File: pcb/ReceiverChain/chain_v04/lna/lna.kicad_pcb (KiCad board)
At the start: 2 copper layers, 40.4 x 15 mm, 17 parts, among them J1 RF-IN, J2 RF-OUT, U1 SKY67159, U2 TPS79933

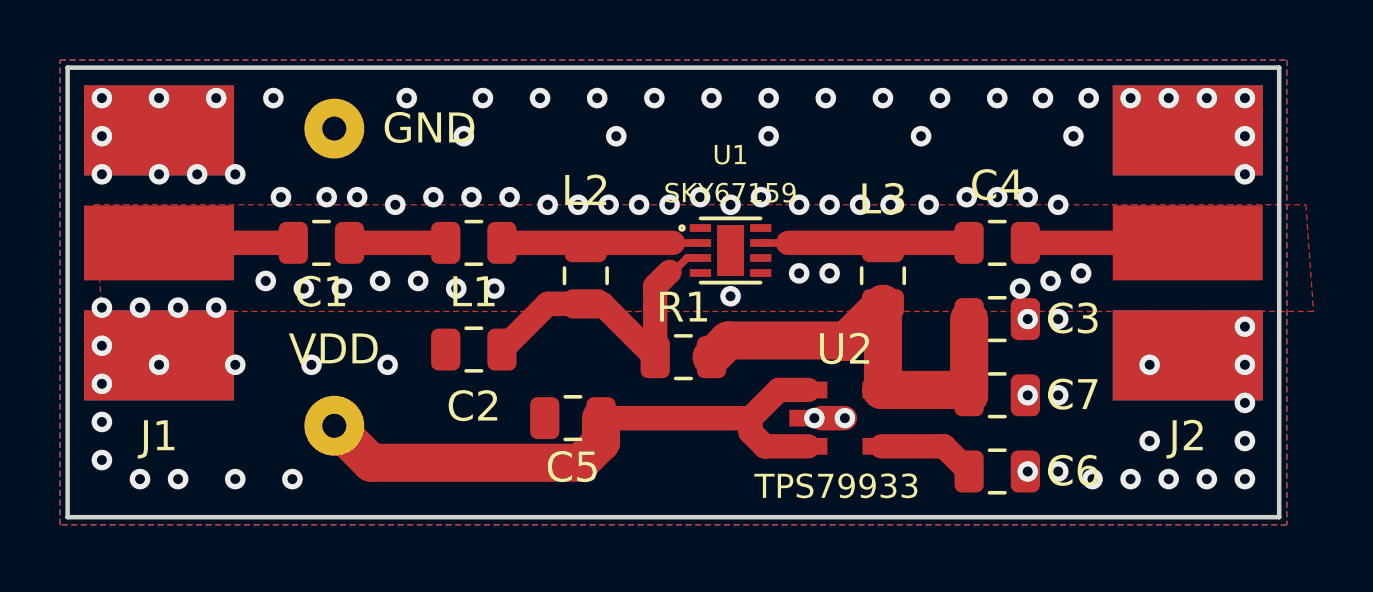
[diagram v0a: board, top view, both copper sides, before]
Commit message: saving
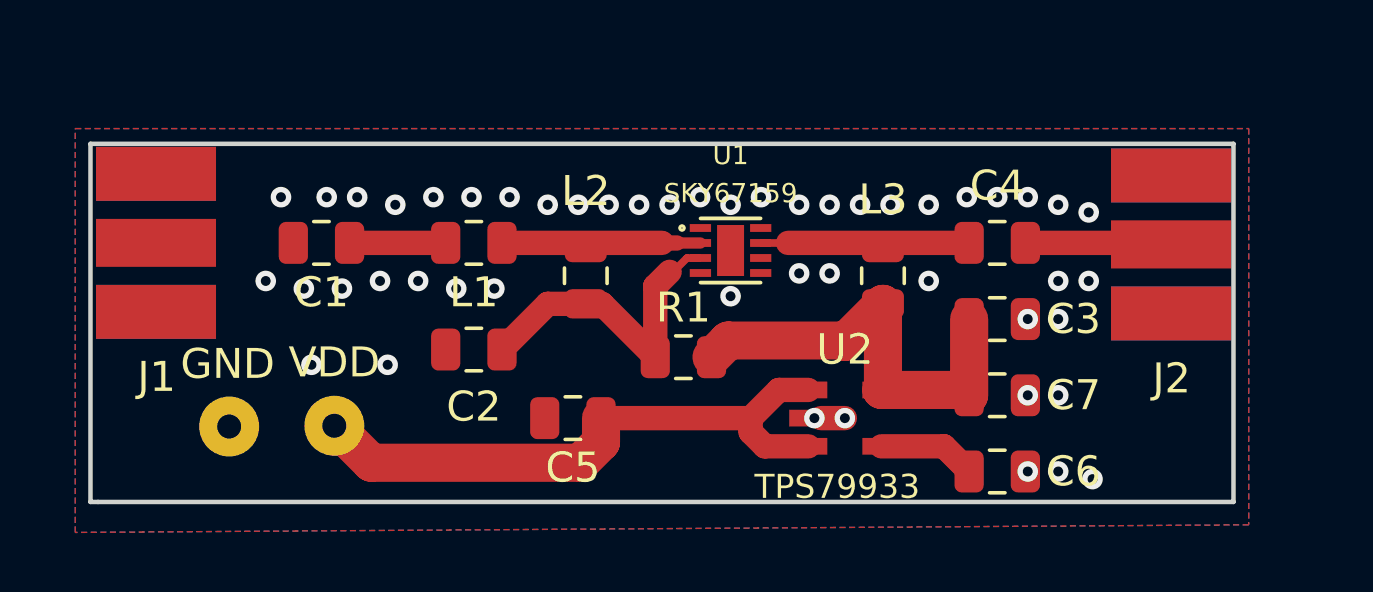
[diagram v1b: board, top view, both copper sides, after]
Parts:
- J1, J2: footprint footprints:SMA-EDGE-16 -> footprints:sma-edge-small
- moved GND 10.5 mm to (76.0, 80.8)
- moved J1 5.25 mm to (73.6, 74.7)
- moved J2 5.23 mm to (107.4, 74.7)
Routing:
- net Net-(C1-Pad2): track 4.49 -> 0.01 mm
- net Net-(C4-Pad1): track 5.41 -> 4.87 mm
- net GND: vias 105 -> 49
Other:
- board size 40.4 x 15 mm -> 38.1 x 11.9 mm
